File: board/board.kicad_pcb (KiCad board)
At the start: 2 copper layers, 37.1 x 49.8 mm, 13 parts, among them J1 Conn_01x19, J2 Conn_01x19, J3 3.3-26V, U1 ESP32-WROVER-E, U2 AOZ1280CI

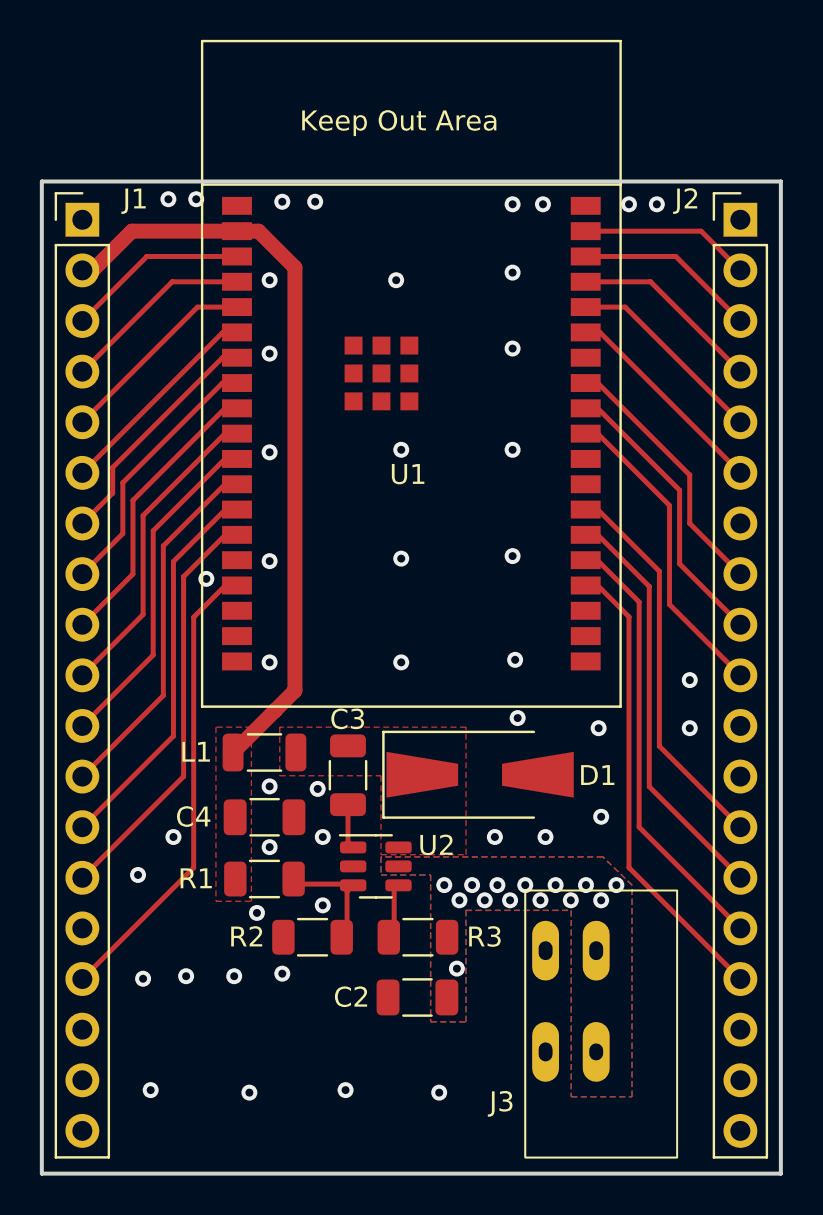
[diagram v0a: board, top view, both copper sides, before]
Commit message: dev
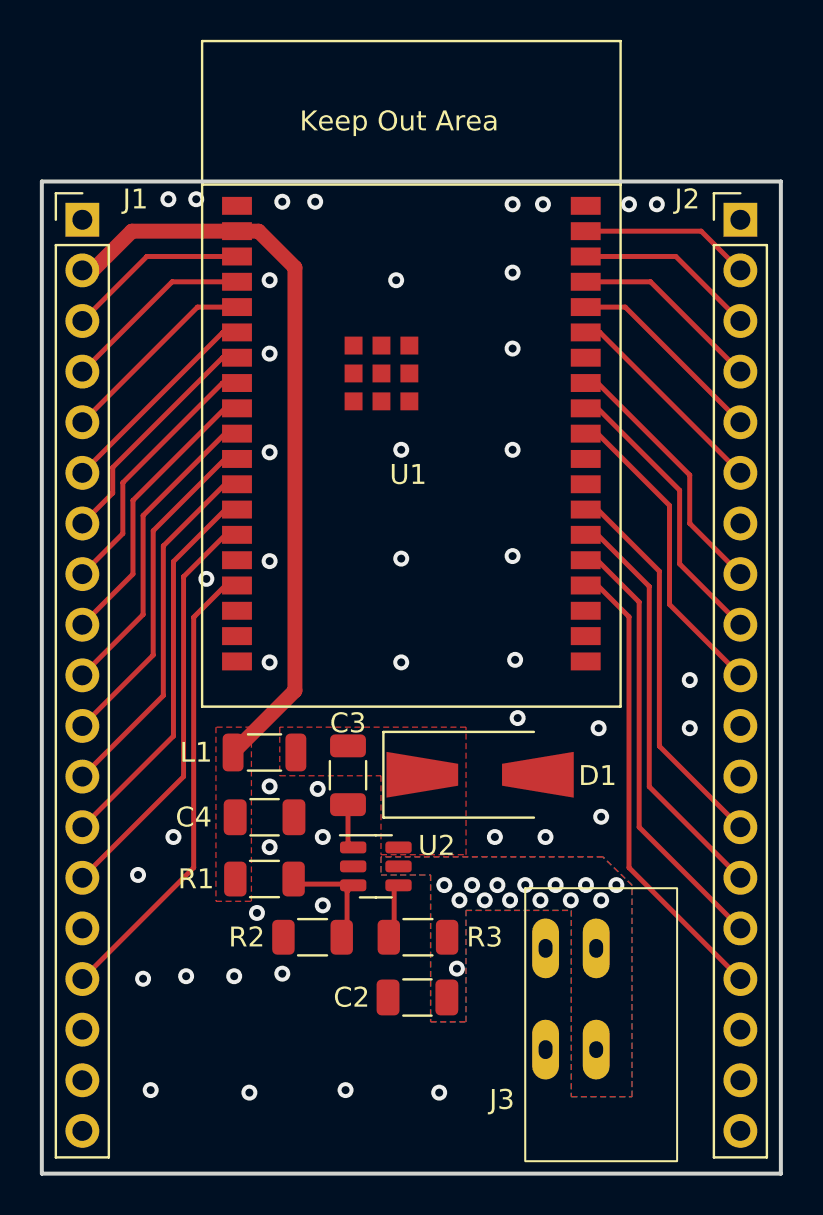
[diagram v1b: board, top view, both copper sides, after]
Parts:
- moved J3 0.12 mm to (159.4, 99.4)
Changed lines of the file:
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@@
     (property "ki_keywords" "capacitor cap")
     (attr smd)
-    (fp_text reference "C3" (at 2.794 0 180) (layer "F.SilkS")
+    (fp_text reference "C3" (at 2.6162 0 180) (layer "F.SilkS")
         (effects (font (size 1 1) (thickness 0.15)))
     )
@@
   )
   (footprint "Custom_Connector:Ninigi AC141R-02P-2.54" (layer "F.Cu")
-    (at 159.385 99.5565)
+    (at 159.385 99.441)
     (property "Sheetfile" "File: board.kicad_sch")
     (property "Sheetname" "")
@@
         (effects (font (size 1 1) (thickness 0.15)))
     )
-    (fp_rect (start 0 -10.64) (end 7.62 2.76)
+    (fp_rect (start 0 -10.64) (end 7.62 3.06)
       (stroke (width 0.1) (type default)) (fill none) (layer "F.SilkS"))
-    (fp_rect (start -0.254 -10.89) (end 7.874 3.032)
+    (fp_rect (start -0.254 -10.89) (end 7.874 3.312)
       (stroke (width 0.05) (type default)) (fill none) (layer "F.CrtYd"))
     (pad "1" thru_hole oval (at 1.02 -7.62) (size 1.35 3) (drill oval 0.7 0.95) (layers *.Cu *.Mask)
@@
   (segment (start 139.6464 55.832) (end 137.6784 57.8) (width 0.75) (layer "F.Cu") (net 3))
   (segment (start 146.002 55.832) (end 144.92 55.832) (width 0.75) (layer "F.Cu") (net 3))
-  (segment (start 146.812 79.90378) (end 146.812 79.883) (width 0.75) (layer "F.Cu") (net 3))
   (segment (start 147.828 78.88778) (end 147.828 57.658) (width 0.75) (layer "F.Cu") (net 3))
   (segment (start 144.92 55.832) (end 139.6464 55.832) (width 0.75) (layer "F.Cu") (net 3))
-  (segment (start 146.8628 79.85298) (end 147.828 78.88778) (width 0.75) (layer "F.Cu") (net 3))
   (segment (start 137.6784 57.8) (end 137.16 57.8) (width 0.75) (layer "F.Cu") (net 3))
-  (segment (start 144.72458 81.9912) (end 146.812 79.90378) (width 0.75) (layer "F.Cu") (net 3))
+  (segment (start 147.828 78.88778) (end 144.72458 81.9912) (width 0.75) (layer "F.Cu") (net 3))
   (segment (start 147.828 57.658) (end 146.002 55.832) (width 0.75) (layer "F.Cu") (net 3))
   (segment (start 144.92 57.102) (end 140.398 57.102) (width 0.25) (layer "F.Cu") (net 4))
